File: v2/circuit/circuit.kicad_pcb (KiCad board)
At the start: 2 copper layers, 90 x 90 mm, 33 parts, among them J1 Conn_01x01, J2 Conn_01x01, J3 Conn_01x01, J4 Conn_01x01, J5 Conn_01x01, M1 Stepper_Motor_bipolar, SW2 SW_Push, U1 ATmega328P-AU, U2 4N25, U3 HT1621B, U4 TSR_1-2450, U5 VIM-878, U6 L293D, U7 FGPMMOPA6H, Y1 Crystal

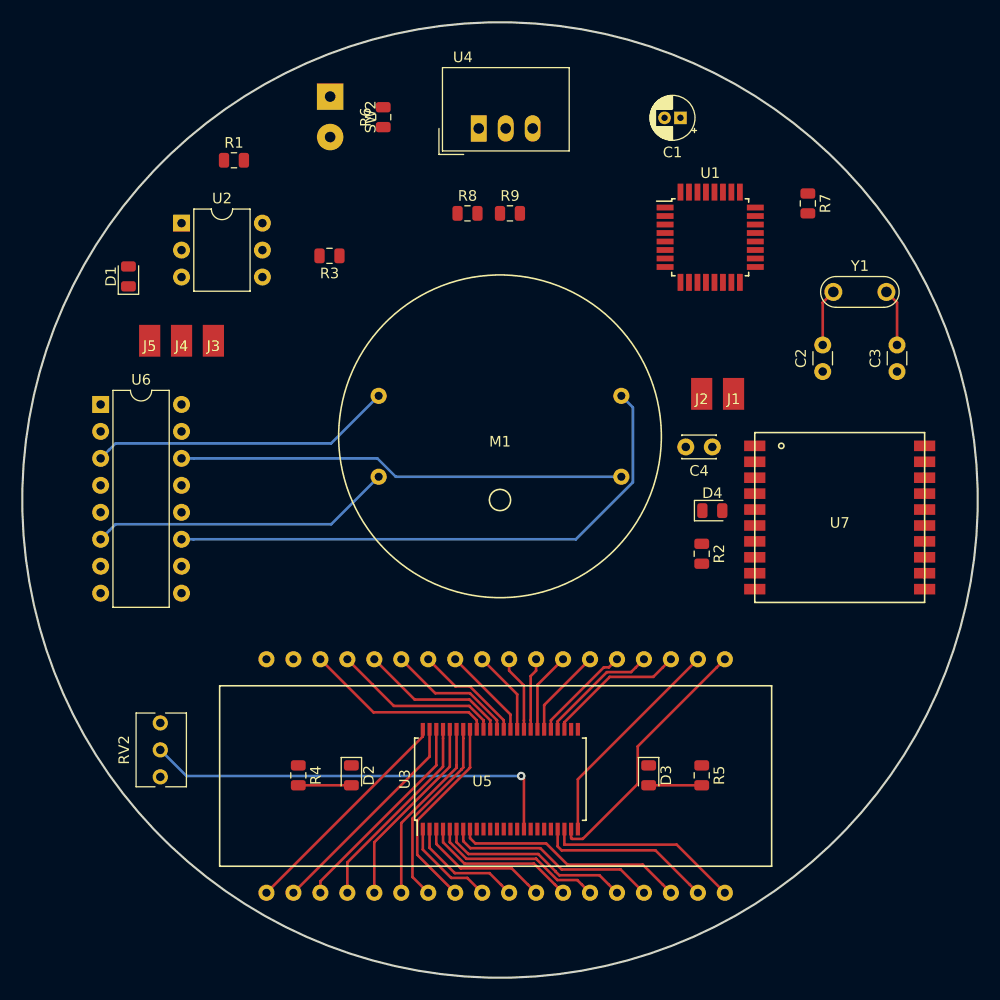
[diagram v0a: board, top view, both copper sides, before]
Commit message: Stuff
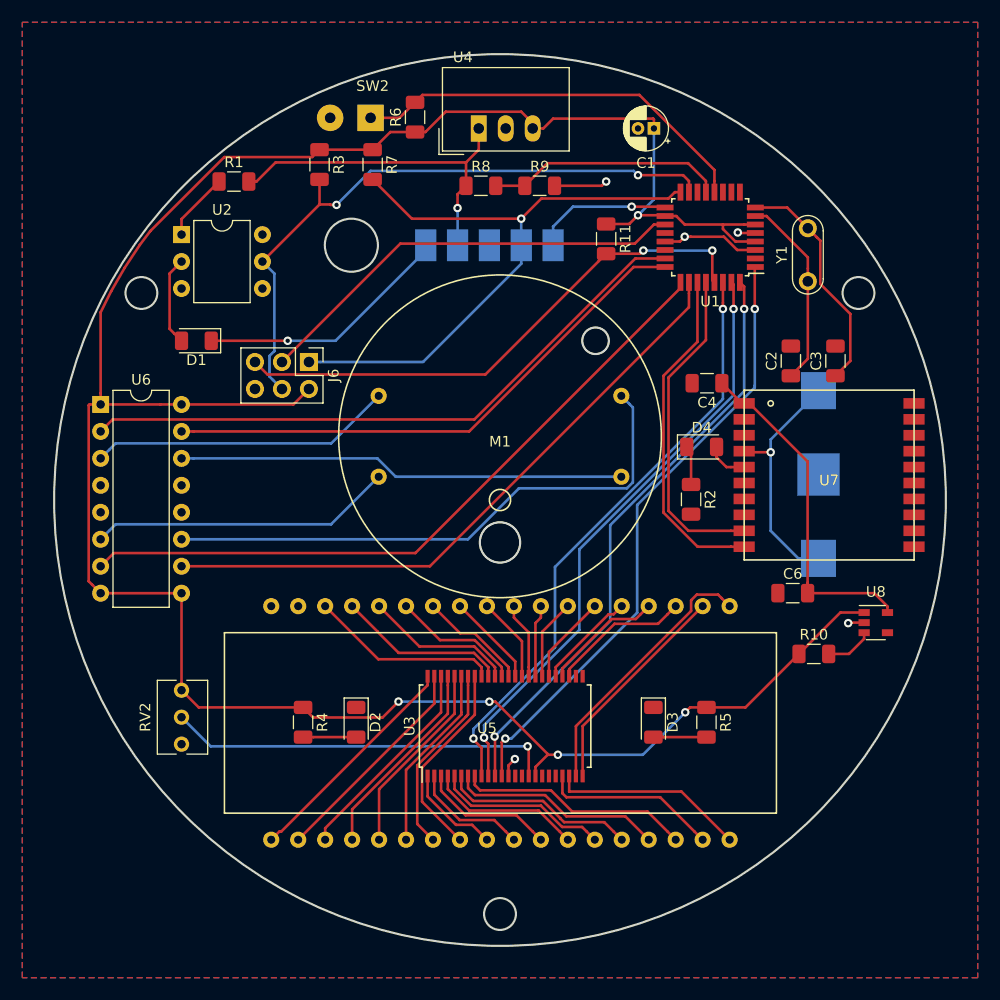
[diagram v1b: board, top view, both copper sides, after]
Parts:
- added BT1: Battery_Cell, Battery:BatteryHolder_Keystone_3000_1x12mm, B.Cu at (180.0, 97.6)
- added C6: C, Capacitor_SMD:C_1206_3216Metric, F.Cu at (177.6, 108.8)
- added J6: Conn_02x03_Odd_Even, Connector_PinHeader_2.54mm:PinHeader_2x03_P2.54mm_Vertical, F.Cu at (132.0, 87.0)
- added R10: R, Resistor_SMD:R_1206_3216Metric, F.Cu at (179.6, 114.5)
- added R11: R, Resistor_SMD:R_1206_3216Metric, F.Cu at (160.0, 75.4)
- added U8: MIC5205-3.3YM5, Package_TO_SOT_SMD:SOT-23-5, F.Cu at (185.4, 111.5)
- C2, C3: value C_Small -> C; footprint Capacitor_THT:C_Disc_D3.0mm_W1.6mm_P2.50mm -> Capacitor_SMD:C_1206_3216Metric
- C4: footprint Capacitor_THT:C_Disc_D3.0mm_W2.0mm_P2.50mm -> Capacitor_SMD:C_1206_3216Metric
- D1, D2, D3, D4: footprint LED_SMD:LED_0805_2012Metric -> LED_SMD:LED_1206_3216Metric
- J1, J2, J3, J4, J5: moved to B.Cu
- R1, R2, R3, R4, R5, R6, R7, R8, R9: footprint Resistor_SMD:R_0805_2012Metric -> Resistor_SMD:R_1206_3216Metric
- moved R7 41.2 mm to (138.0, 68.4)
- moved J5 33.2 mm to (149.0, 76.0)
- moved J4 27.5 mm to (146.0, 76.0)
- moved J1 24.4 mm to (152.0, 76.0)
- moved J3 21.9 mm to (143.0, 76.0)
- moved J2 19.8 mm to (155.0, 76.0)
- moved D1 8.82 mm to (121.4, 85.0), turned to 180 degrees
- moved R3 8.65 mm to (133.0, 68.4), turned to 270 degrees
- moved D4 6.08 mm to (169.0, 95.0)
- moved C4 6.02 mm to (169.5, 89.0)
- moved C3 5.89 mm to (181.6, 86.9)
- moved R2 5.22 mm to (168.0, 99.9)
- moved D2 5.02 mm to (136.4, 120.9)
- moved D3 5.02 mm to (164.4, 120.9)
- moved R4 5.02 mm to (131.4, 120.9)
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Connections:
- C2 pad 1: GND -> /XTAL1
- C2 pad 2: /XTAL1 -> GND
- C3 pad 1: GND -> /XTAL2
- C3 pad 2: /XTAL2 -> GND
- U1 pad 14: /AFR -> (no net)
- U1 pad 17: (no net) -> /AFR
- U1 pad 19: (no net) -> Net-(J6-Pad3)
- U1 pad 27: (no net) -> /RX
- U1 pad 28: (no net) -> /TX
- U1 pad 29: +5V -> Net-(J6-Pad5)
- U6 pad 10: /STEP_3 -> /STEP_4
- U6 pad 15: /STEP_4 -> /STEP_2
- U6 pad 7: /STEP_2 -> /STEP_3
- U7 pad 10: (no net) -> /RX
- U7 pad 4: (no net) -> /VBACKUP
- U7 pad 9: (no net) -> /TX
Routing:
- net +5V: track 0.00 -> 231.9 mm, vias 0 -> 5
- net /STEP_3: track 0.00 -> 66.0 mm
- net /TACHO: track 0.00 -> 60.7 mm, vias 0 -> 2
- net /STEP_4: track 0.00 -> 60.2 mm
- net /OIL_TEMP: track 0.00 -> 60.1 mm, vias 0 -> 1
- net /STEP_1: track 0.00 -> 59.9 mm
- net /LCD_DATA: track 0.00 -> 58.2 mm, vias 0 -> 2
- net /LCD_CS: track 0.00 -> 56.5 mm, vias 0 -> 2
- net /LCD_RD: track 0.00 -> 56.5 mm, vias 0 -> 2
- net /LCD_WR: track 0.00 -> 56.4 mm, vias 0 -> 2
- net /STEP_2: track 0.00 -> 52.0 mm
- net Net-(J6-Pad5): track 0.00 -> 51.5 mm, vias 0 -> 2
- net Net-(J6-Pad3): track 0.00 -> 41.5 mm
- net /MODE_BUTTON: track 0.00 -> 38.3 mm
- net +12V: track 0.00 -> 33.0 mm, vias 0 -> 1
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- added copper zone on B.Cu, net GND
- added copper zone on F.Cu, net GND
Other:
- board size 90 x 90 mm -> 84 x 84 mm
- board text added: "12V"
- board text added: "AFR"
- board text added: "GND"
- board text added: "OIL TEMP"
- board text added: "TACHO"
